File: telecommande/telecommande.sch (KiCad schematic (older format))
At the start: 43 parts, among them J1 Conn_01x08_Male, J2 Conn_01x02_Male, J3 Conn_01x04_Male, J4 Conn_01x04_Male, J5 Conn_01x06_Male, J6 Screw_Terminal_01x02, J7 Screw_Terminal_01x02, J8 Conn_01x01_Male, K1 ATX203, Q1 BS170, SW1 SW_MEC_5E, U1 L78L05_TO92, U2 PIC18F26K80_ISS, U3 24LC1026-I_P, U4 L7812, Y1 Crystal 16MHz

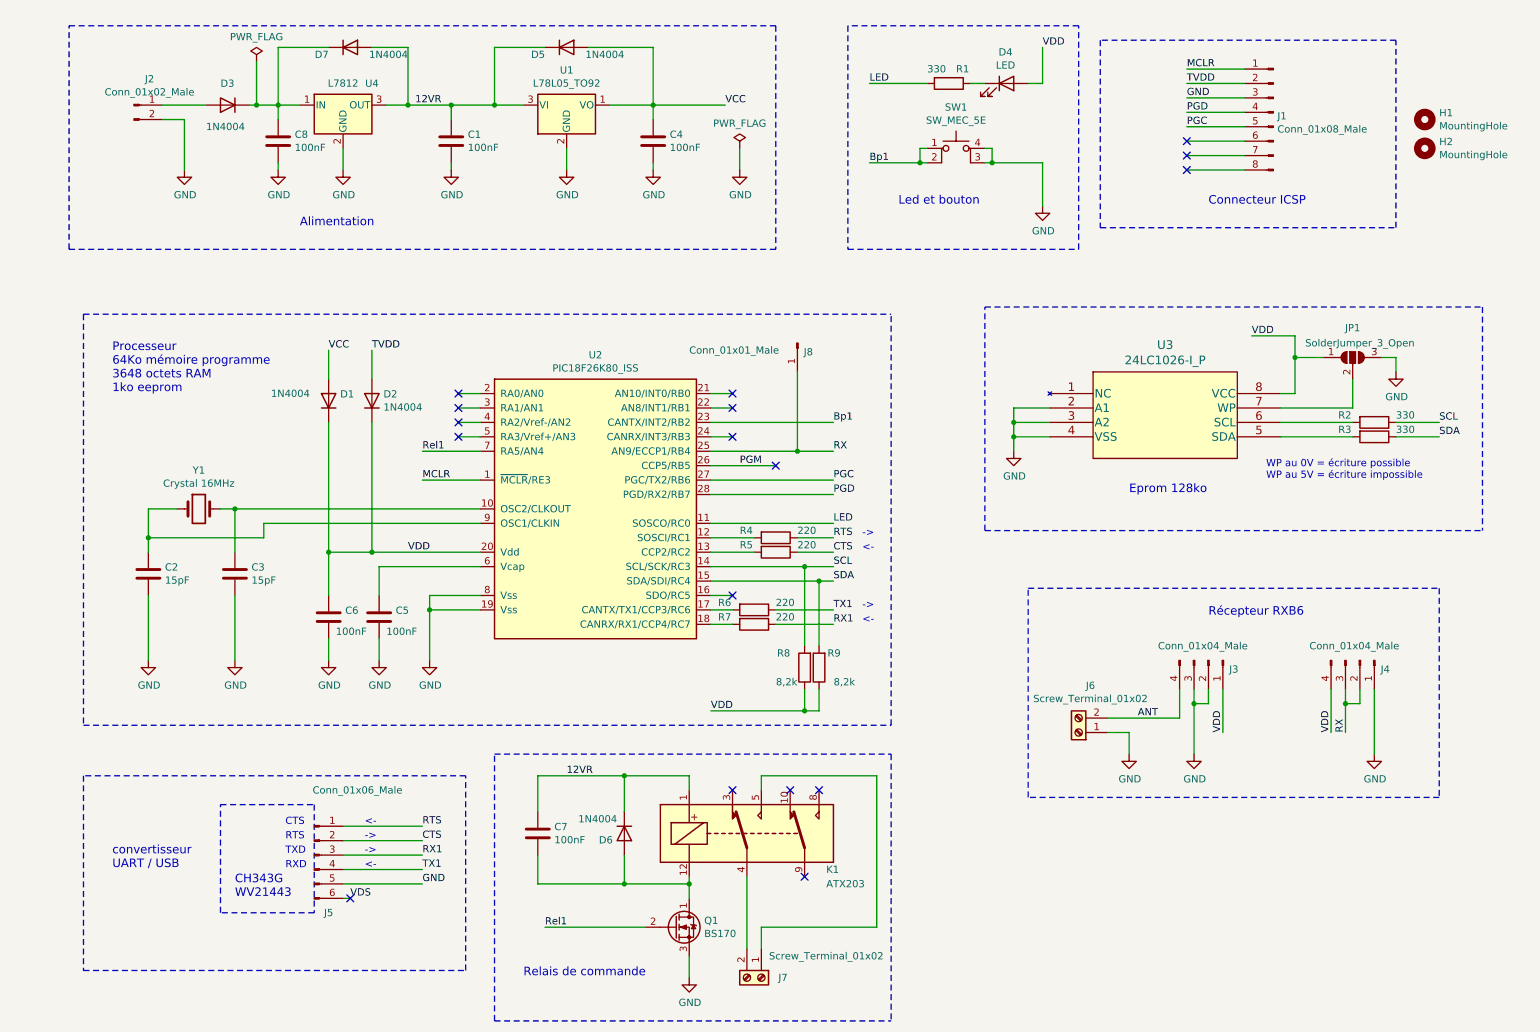
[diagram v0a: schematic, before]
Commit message: add came
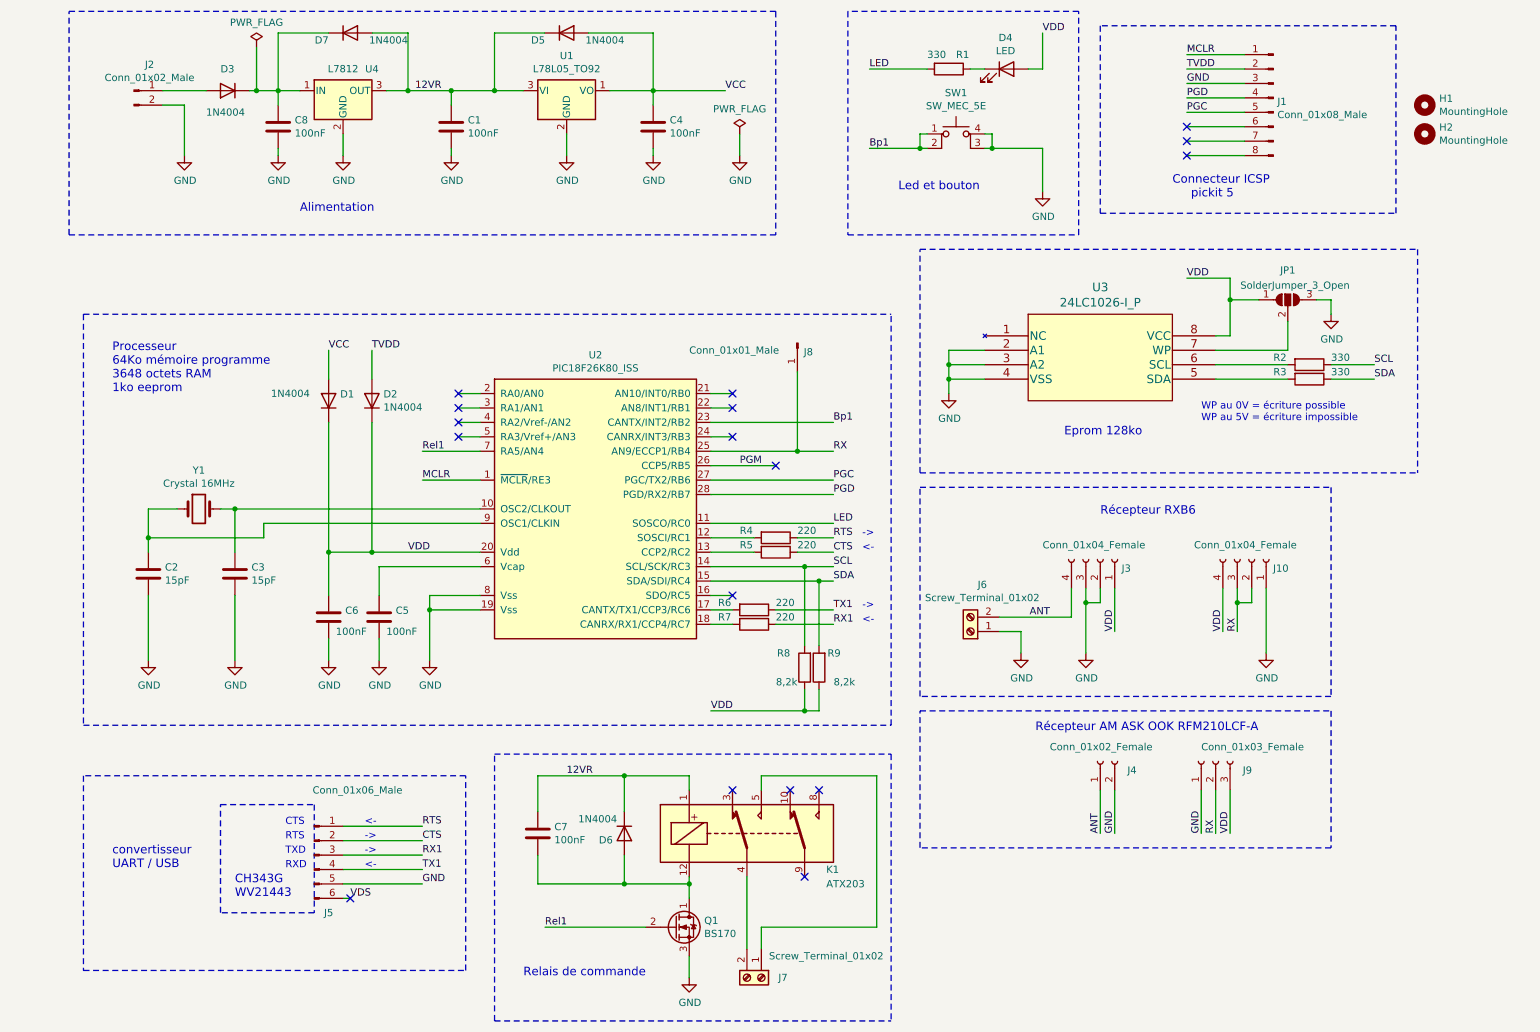
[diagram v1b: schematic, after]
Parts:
- removed J3, J4: Conn_01x04_Male, Connector_PinSocket_2.54mm:PinSocket_1x04_P2.54mm_Vertical, symbol Connector:Conn_01x04_Male
- added J10, J3: Conn_01x04_Female, Connector_PinSocket_2.54mm:PinSocket_1x04_P2.54mm_Vertical, symbol Connector:Conn_01x04_Female
- added J4: Conn_01x02_Female, Connector_PinSocket_2.54mm:PinSocket_1x02_P2.54mm_Vertical, symbol Connector:Conn_01x02_Female
- added J9: Conn_01x03_Female, Connector_PinSocket_2.54mm:PinSocket_1x03_P2.54mm_Vertical, symbol Connector:Conn_01x03_Female
- D3: footprint Diode_THT:D_DO-41_SOD81_P10.16mm_Horizontal -> Diode_THT:D_DO-41_SOD81_P7.62mm_Horizontal
- J2: footprint Connector_PinSocket_2.54mm:PinSocket_1x02_P2.54mm_Vertical -> Connector_PinHeader_2.54mm:PinHeader_1x02_P2.54mm_Vertical
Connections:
- net ANT: now also J3.4 (Pin_4), J4.1 (Pin_1)
- net GND: now also J10.1 (Pin_1), J3.2 (Pin_2), J3.3 (Pin_3), J4.2 (Pin_2), J9.1 (Pin_1)
- net RX: now also J10.2 (Pin_2), J10.3 (Pin_3), J9.2 (Pin_2)
- net VDD: now also J10.4 (Pin_4), J3.1 (Pin_1), J9.3 (Pin_3)
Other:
- note added: "Connecteur ICSP\n pickit 5"
- note added: "Récepteur AM ASK OOK RFM210LCF-A"
- note removed: "Connecteur ICSP"
- moved on the sheet: C1, C4, C8, D3, D4, D5, D7, H1, H2, J1, J2, J6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

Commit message: V2
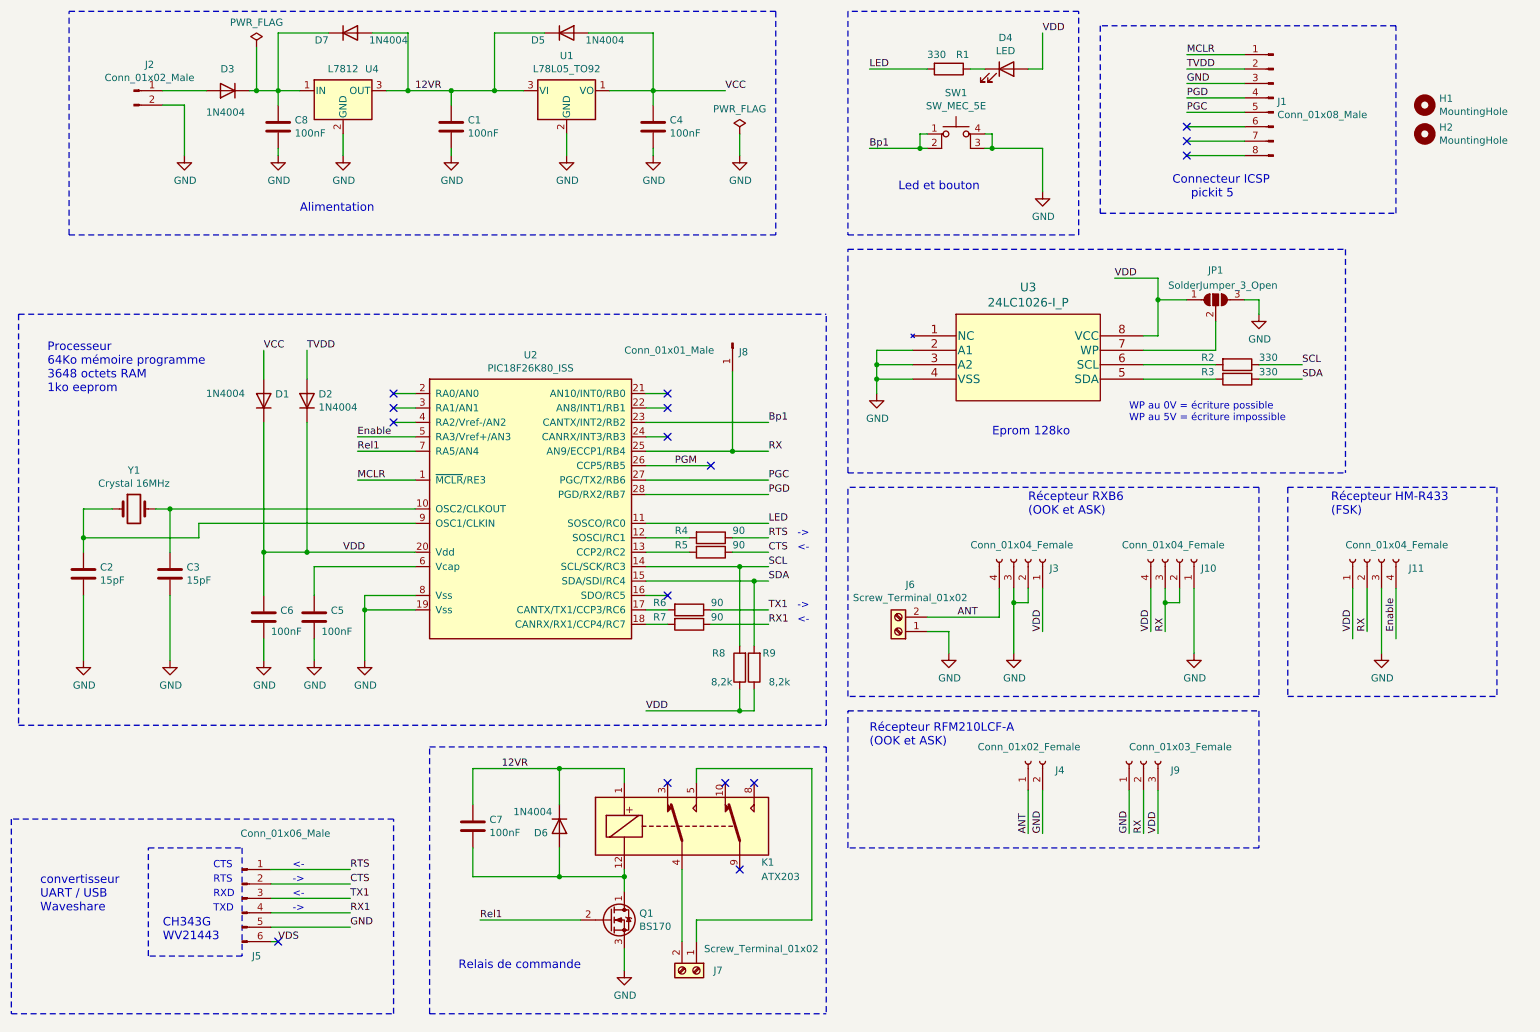
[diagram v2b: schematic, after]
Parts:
- added J11: Conn_01x04_Female, Connector_PinSocket_2.54mm:PinSocket_1x04_P2.54mm_Vertical, symbol Connector:Conn_01x04_Female
- R4, R5, R6, R7: value 220 -> 90
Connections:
- net GND: now also J11.3 (Pin_3)
- net RX: now also J11.2 (Pin_2)
- net RX1: now also J5.4 (Pin_4); no longer J5.3 (Pin_3)
- net TX1: now also J5.3 (Pin_3); no longer J5.4 (Pin_4)
- net VDD: now also J11.1 (Pin_1)
- net Enable: now reaches U2.5 (RA3/Vref+/AN3)
- net Enable: now also J11.4 (Pin_4)
- no-connect marks 17 -> 16
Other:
- note added: "Récepteur HM-R433 \n(FSK)\n"
- note added: "Récepteur RFM210LCF-A\n(OOK et ASK)"
- note added: "Récepteur RXB6\n(OOK et ASK)"
- note added: "convertisseur\nUART / USB\nWaveshare"
- note removed: "Récepteur AM ASK OOK RFM210LCF-A"
- note removed: "Récepteur RXB6"
- note removed: "convertisseur\nUART / USB"
- moved on the sheet: C2, C3, C5, C6, C7, D1, D2, D6, J10, J3, J4, J5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
